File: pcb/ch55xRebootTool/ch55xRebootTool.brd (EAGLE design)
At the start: 40.6 x 33 mm, 32 parts, among them IC1 CH443K, IC2 CH443K, IC3 74AHCT1G08DCK, U2 CH552G

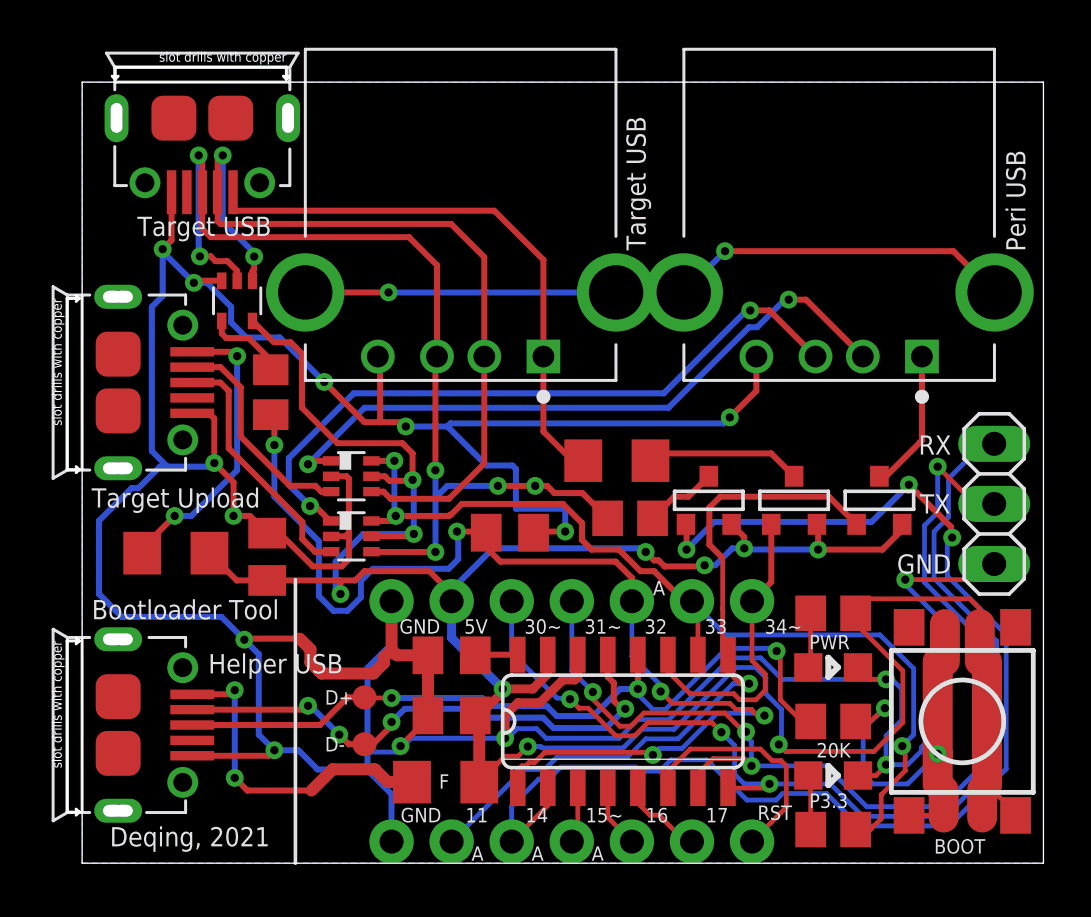
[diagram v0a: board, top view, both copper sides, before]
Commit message: update PCB and separate VCC
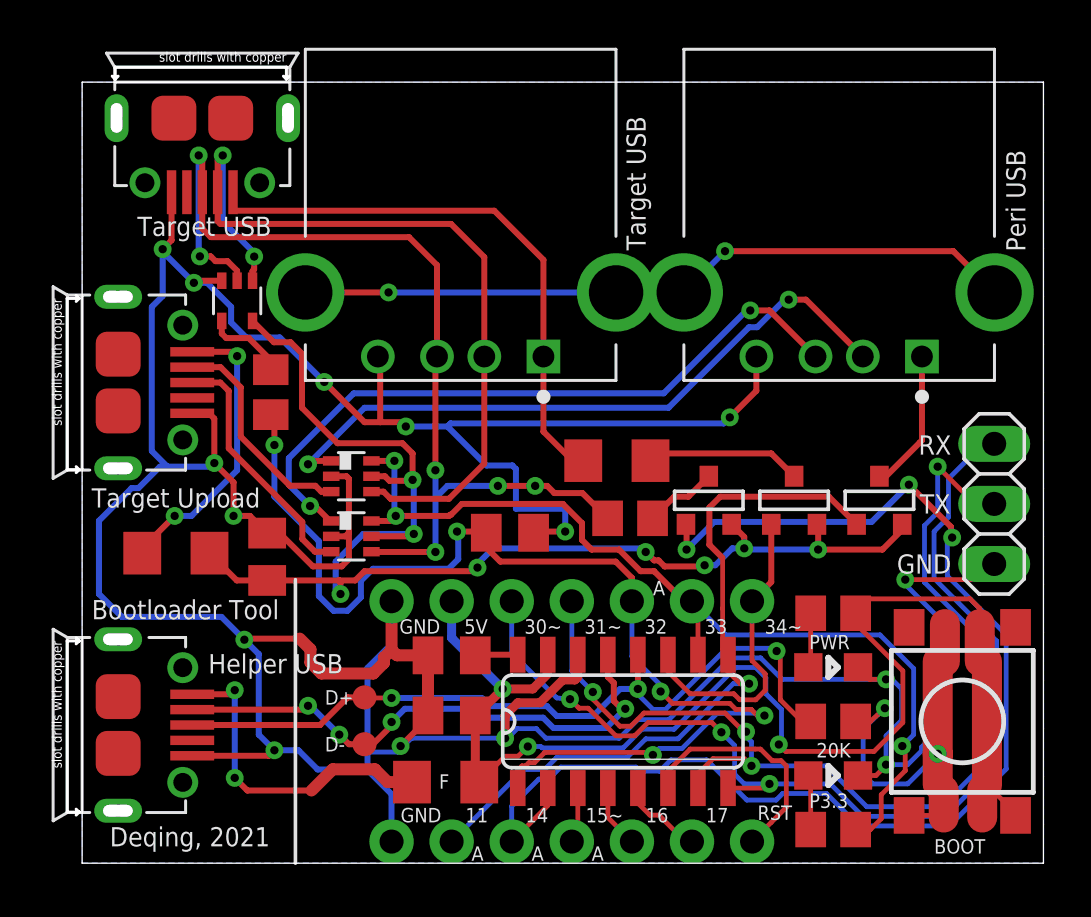
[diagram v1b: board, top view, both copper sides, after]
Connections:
- new net VCC: C1.1, F1.2, J2.2, R2.1, S1.B2, U2.15
- net +5V: no longer C1.1, F1.2, J2.2, R2.1, S1.B2, U2.15
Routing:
- net +5V: track 116.7 -> 57.4 mm, vias 10 -> 8
- net VCC: track 0.00 -> 58.5 mm, vias 0 -> 3
